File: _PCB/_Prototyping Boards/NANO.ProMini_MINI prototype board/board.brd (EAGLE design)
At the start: 57.2 x 41 mm, 27 parts, among them T1_5MM 5mm

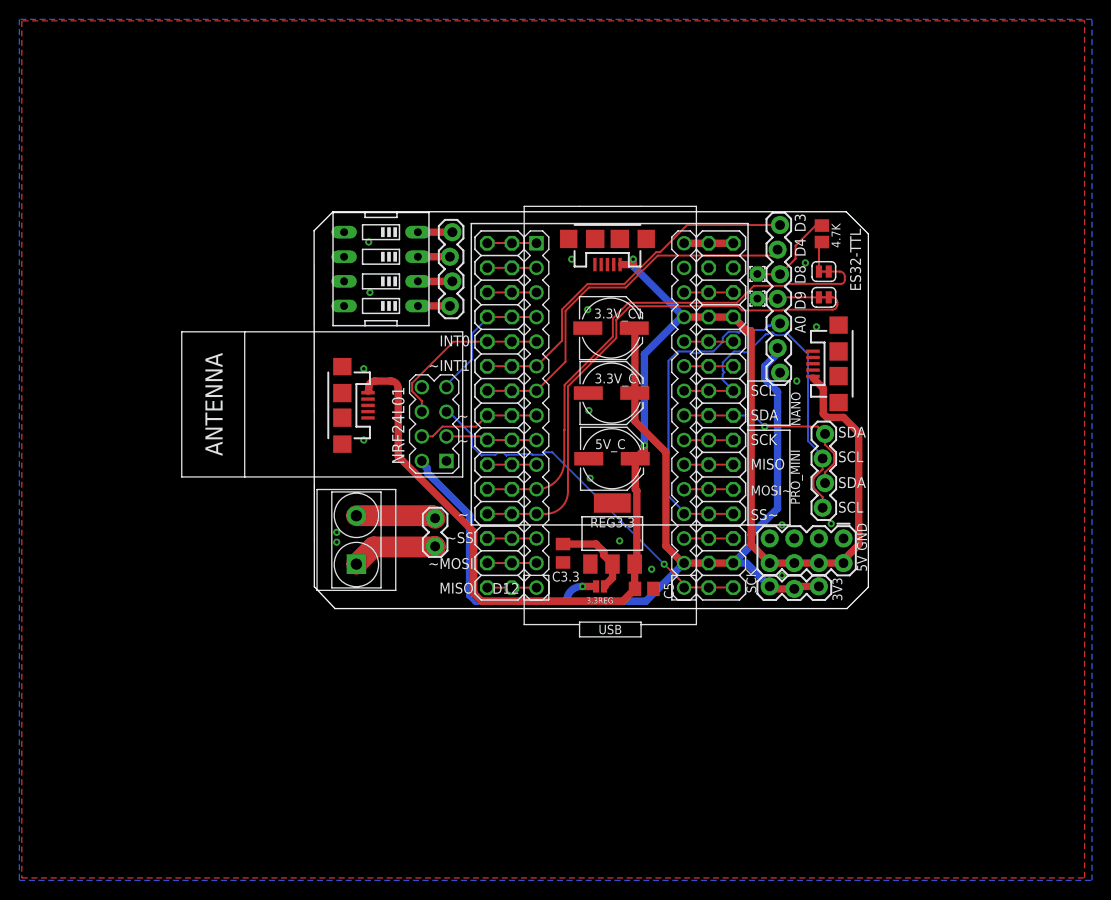
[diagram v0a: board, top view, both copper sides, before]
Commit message: PCB update
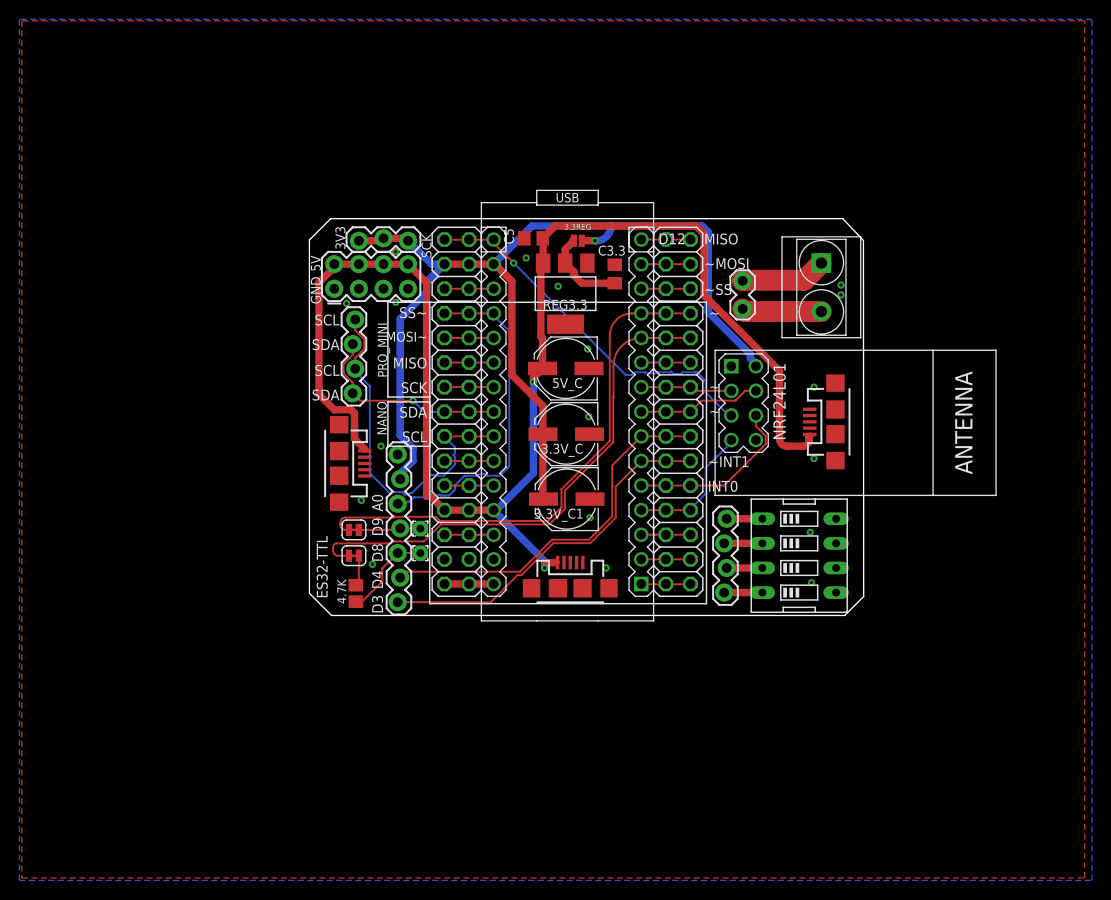
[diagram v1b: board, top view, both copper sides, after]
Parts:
- moved R1 60.8 mm to (4.26, 1.69), turned to 270 degrees
- moved JP1 56.7 mm to (4.06, 5.59), turned to 0 degrees
- moved ES32-TTL 55.3 mm to (8.71, 0.79), turned to 90 degrees
- moved NRF24L01 54.9 mm to (55.7, 18.8), turned to 0 degrees
- moved T1_5MM 54.6 mm to (52.3, 33.3), turned to 0 degrees
- moved JP2 54.1 mm to (4.06, 8.26), turned to 0 degrees
- moved 5.GND 53.1 mm to (5.84, 34.4), turned to 0 degrees
- moved MICRO_3 52.6 mm to (2.54, 15.1), turned to 180 degrees
- moved SW1 52.3 mm to (50.0, 5.59), turned to 270 degrees
- moved I2C_1 52.3 mm to (4.06, 30.0), turned to 270 degrees
- moved 3V3 51.8 mm to (9.65, 38.2), turned to 180 degrees
- moved MICRO_1 50.9 mm to (53.8, 19.4), turned to 0 degrees
- moved J4 46.8 mm to (42.4, 1.78), turned to 90 degrees
- moved PAD2 45.2 mm to (10.9, 5.84), turned to 180 degrees
- moved PAD1 42.1 mm to (10.9, 8.38), turned to 180 degrees
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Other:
- outline, holes or cut-outs redrawn
